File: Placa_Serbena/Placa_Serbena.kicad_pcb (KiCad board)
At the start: 2 copper layers, 34 parts

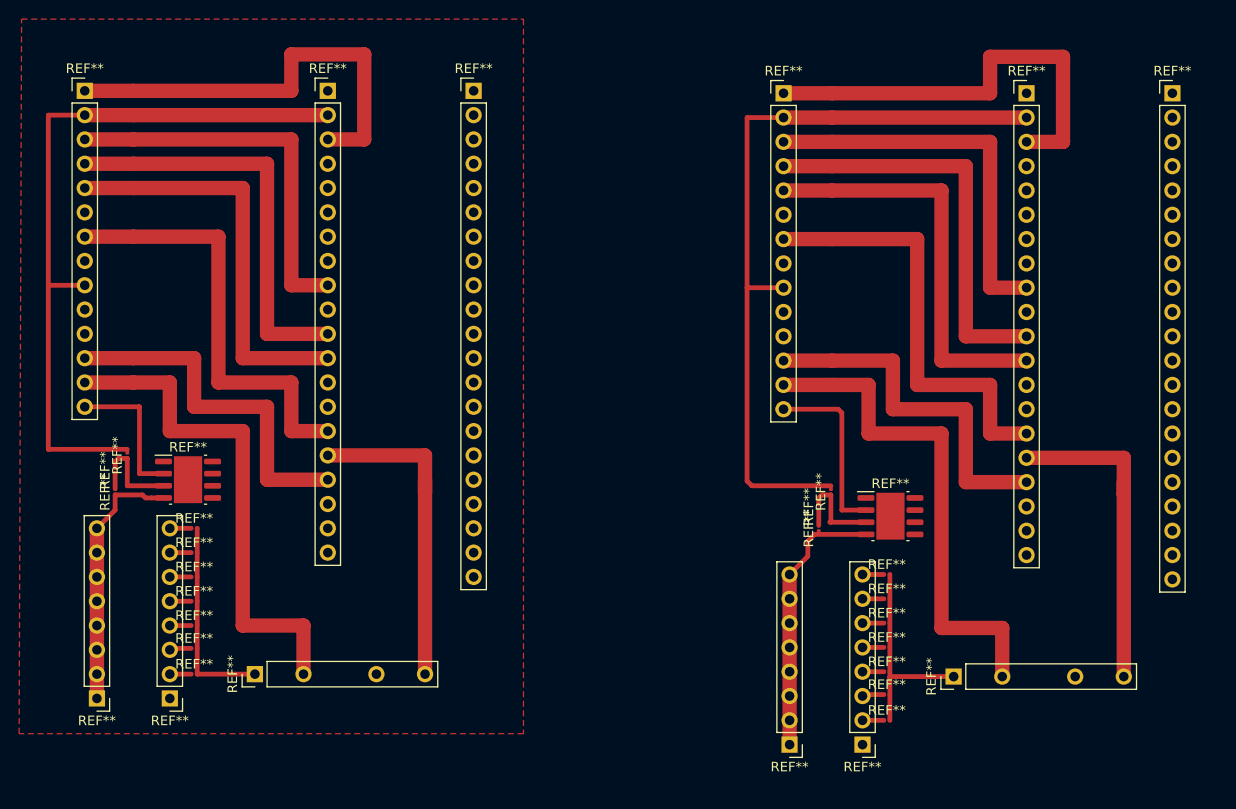
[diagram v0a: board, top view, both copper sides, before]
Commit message: Amplificador check
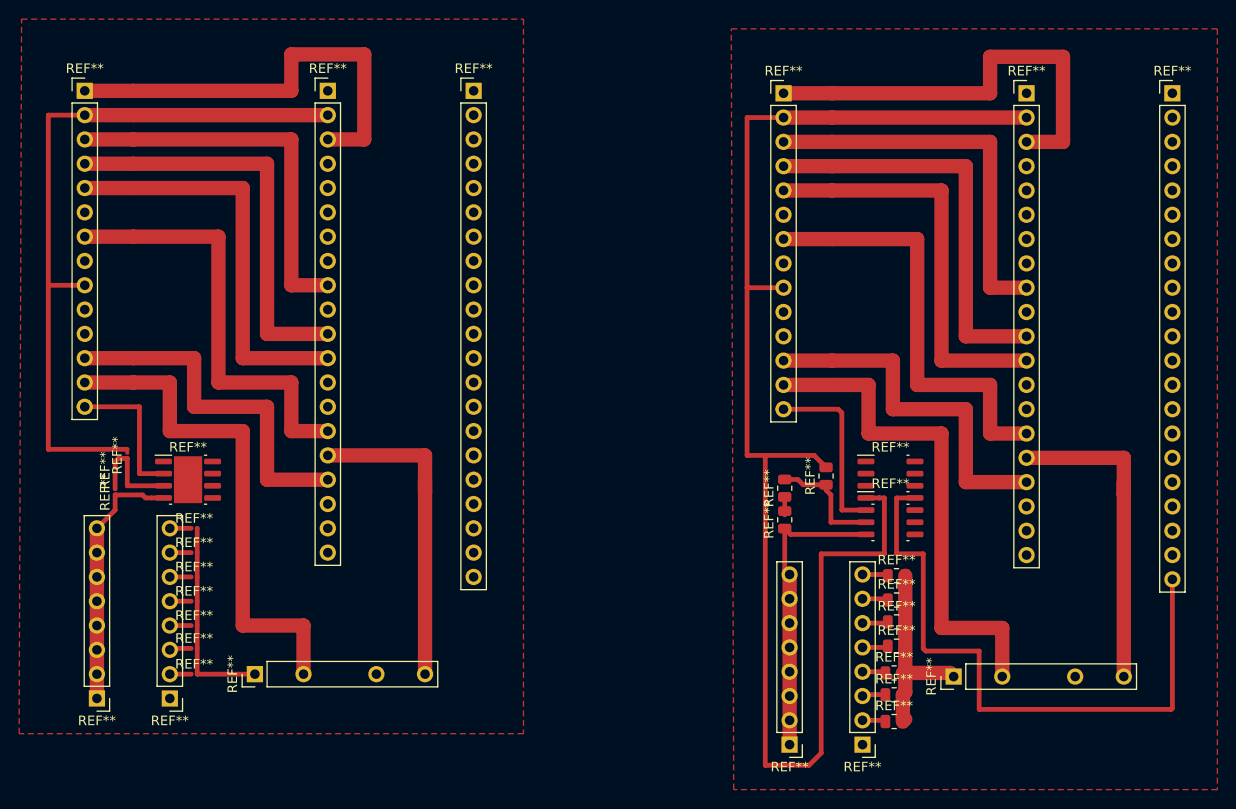
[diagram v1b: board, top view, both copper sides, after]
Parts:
- removed the REF** at (126.2, 100.6)
- removed the REF** at (126.2, 95.6)
- removed the REF** at (126.2, 103.3)
- removed the REF** at (120.4, 79.4)
- removed the REF** at (126.2, 93.1)
- removed the REF** at (126.2, 90.6)
- removed the REF** at (119.1, 80.9)
- removed the REF** at (126.2, 88.0)
- removed the REF** at (126.2, 98.2)
- removed the REF** at (119.1, 83.2)
- added REF**: R_0805_2012Metric, Resistor_SMD:R_0805_2012Metric, F.Cu at (127.0, 103.4)
- added REF**: R_0805_2012Metric, Resistor_SMD:R_0805_2012Metric, F.Cu at (127.3, 90.7)
- added REF**: R_0805_2012Metric, Resistor_SMD:R_0805_2012Metric, F.Cu at (127.3, 88.1)
- added REF**: R_0805_2012Metric, Resistor_SMD:R_0805_2012Metric, F.Cu at (115.6, 79.0)
- added REF**: R_0805_2012Metric, Resistor_SMD:R_0805_2012Metric, F.Cu at (115.6, 82.3)
- added REF**: R_0805_2012Metric, Resistor_SMD:R_0805_2012Metric, F.Cu at (119.9, 77.7)
- added REF**: R_0805_2012Metric, Resistor_SMD:R_0805_2012Metric, F.Cu at (127.0, 100.6)
- added REF**: R_0805_2012Metric, Resistor_SMD:R_0805_2012Metric, F.Cu at (127.0, 98.3)
- added REF**: R_0805_2012Metric, Resistor_SMD:R_0805_2012Metric, F.Cu at (127.3, 95.5)
- added REF**: R_0805_2012Metric, Resistor_SMD:R_0805_2012Metric, F.Cu at (127.3, 93.0)
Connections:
- REF** pad 1: (no net) -> GNDREF
- REF** pad 4: (no net) -> GNDREF
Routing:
- net (no net): track 874.4 -> 947.0 mm
- net GNDREF: track 156.2 -> 227.4 mm
